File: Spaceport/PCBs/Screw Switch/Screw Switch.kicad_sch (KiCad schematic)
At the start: 3 parts

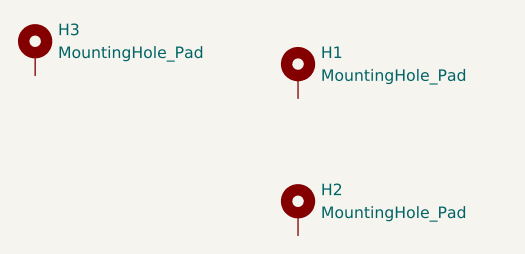
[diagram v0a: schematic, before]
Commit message: Revert "Merge branch 'main' of https://github.com/Terrapin-Rocket-Team/SRAD-Avionics"
This reverts commit e5f68e4e525f2a5ad7eebbc917cc2807b67ca5e1, reversing
changes made to 8a40e2e341d8980ca528983581171a8bd9cc0146.
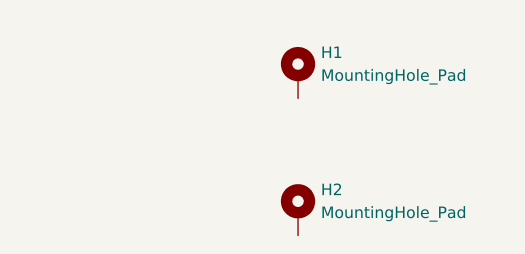
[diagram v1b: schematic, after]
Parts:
- removed H3: MountingHole_Pad, MountingHole:MountingHole_3.2mm_M3_Pad_TopBottom, symbol Mechanical:MountingHole_Pad
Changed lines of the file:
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@@
-	(symbol
-		(lib_id "Mechanical:MountingHole_Pad")
-		(at 82.55 68.58 0)
-		(unit 1)
-		(exclude_from_sim yes)
-		(in_bom no)
-		(on_board yes)
-		(dnp no)
-		(fields_autoplaced yes)
-		(property "Reference" "H3"
-			(at 85.09 66.0399 0)
-			(effects
-				(font
-					(size 1.27 1.27)
-				)
-				(justify left)
-			)
-		)
-		(property "Value" "MountingHole_Pad"
-			(at 85.09 68.5799 0)
-			(effects
-				(font
-					(size 1.27 1.27)
-				)
-				(justify left)
-			)
-		)
-		(property "Footprint" "MountingHole:MountingHole_3.2mm_M3_Pad_TopBottom"
-			(at 82.55 68.58 0)
-			(effects
-				(font
-					(size 1.27 1.27)
-				)
-				(hide yes)
-			)
-		)
-		(property "Datasheet" "~"
-			(at 82.55 68.58 0)
-			(effects
-				(font
-					(size 1.27 1.27)
-				)
-				(hide yes)
-			)
-		)
-		(property "Description" "Mounting Hole with connection"
-			(at 82.55 68.58 0)
-			(effects
-				(font
-					(size 1.27 1.27)
-				)
-				(hide yes)
-			)
-		)
-		(pin "1"
-		)
-		(instances
-			(project "Screw Switch"
-				(path "/95d75f6d-4b6e-4fd0-917d-ccbce393357a"
-					(reference "H3")
-					(unit 1)
-				)
-			)
-		)
-	)
 	(symbol
 		(lib_id "Mechanical:MountingHole_Pad")
